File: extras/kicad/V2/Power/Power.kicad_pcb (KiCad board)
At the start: 2 copper layers, 181.3 x 110 mm, 90 parts, among them J1 Conn_01x02, J2 Screw_Terminal_01x06, J3 Screw_Terminal_01x06, J4 Screw_Terminal_01x06, J5 Screw_Terminal_01x06, J6 left, J7 right, SW1 SW_SPST, U1 TB6612FNG, U2 TB6612FNG, U3 TPS5430DDAR, U4 TPS5430DDAR, U5 INA219AxD

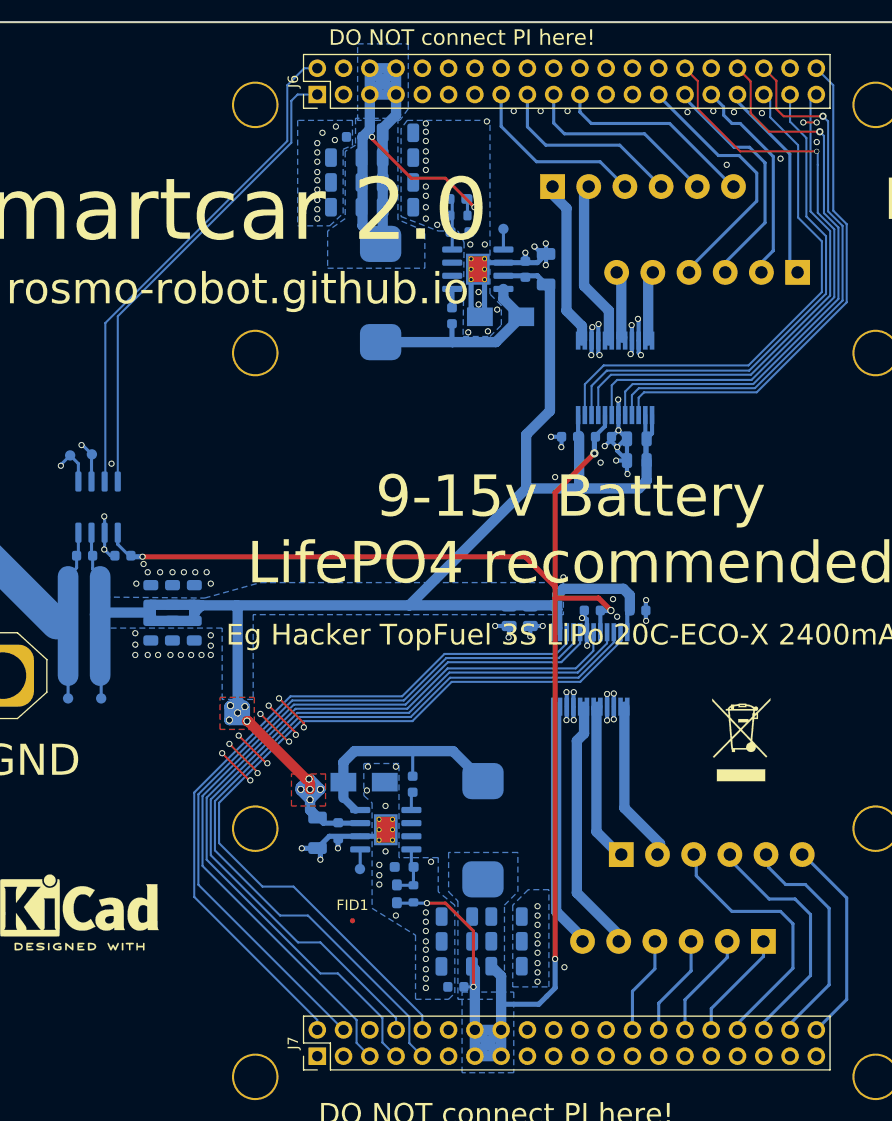
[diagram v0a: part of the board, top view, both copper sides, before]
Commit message: m
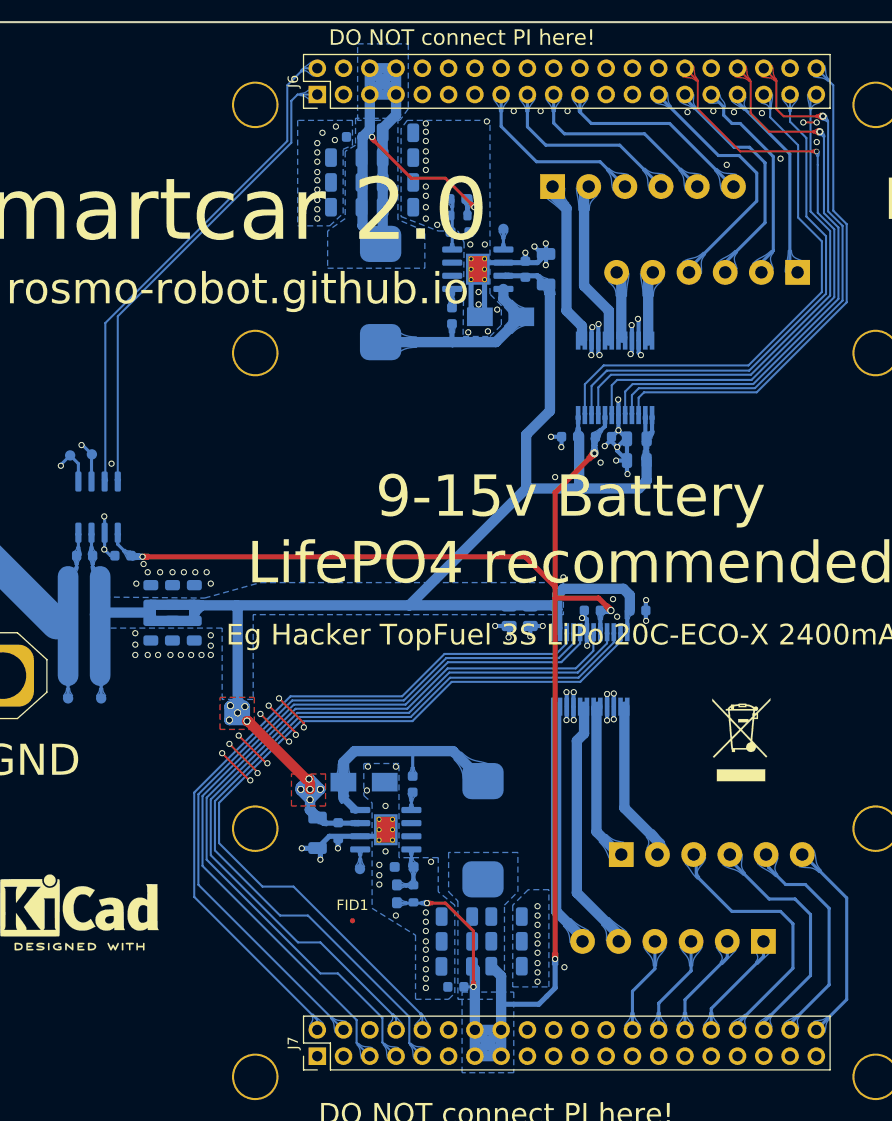
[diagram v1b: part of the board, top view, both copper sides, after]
